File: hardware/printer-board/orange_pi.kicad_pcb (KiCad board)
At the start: 2 copper layers, 12 parts, among them J1 USB_DEBUG, U1 orange_pi_zero

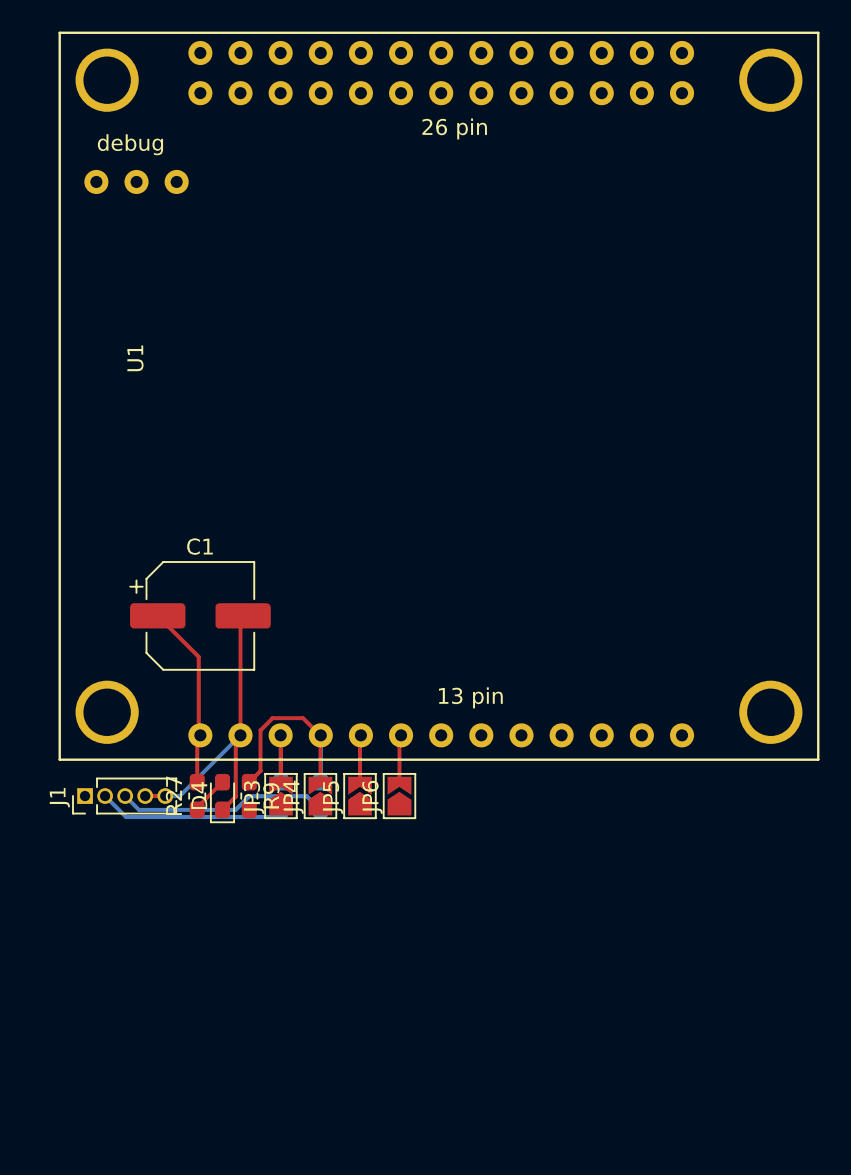
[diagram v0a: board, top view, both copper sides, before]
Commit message: update,
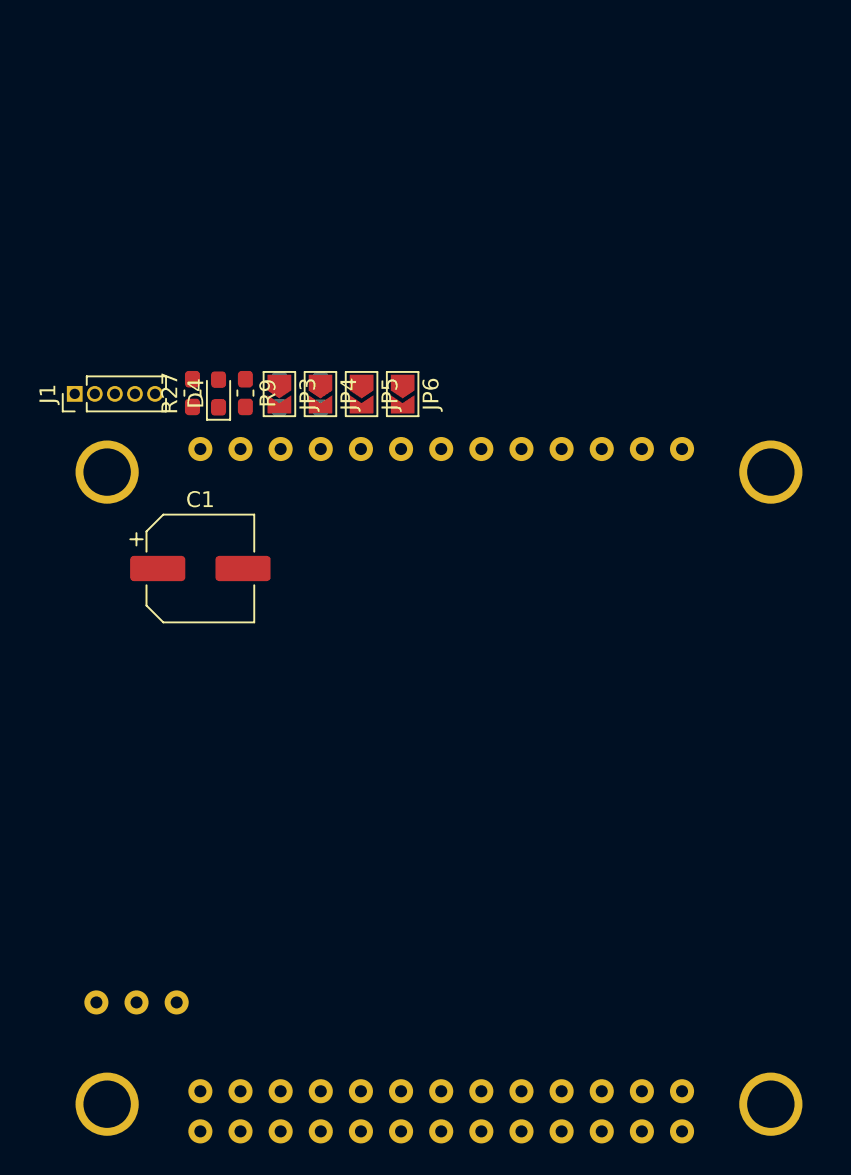
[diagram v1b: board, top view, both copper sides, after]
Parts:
- U1: moved to B.Cu
- moved R27 25.5 mm to (40.5, 46.4)
- moved R9 25.5 mm to (43.9, 46.4)
- moved D4 25.5 mm to (42.1, 46.4)
- moved J1 25.5 mm to (33.0, 46.5)
- moved R5 25.5 mm to (46.0, 46.4), turned to 90 degrees
- moved JP6 25.4 mm to (53.8, 46.5), turned to 270 degrees
- moved JP5 25.4 mm to (51.2, 46.5), turned to 270 degrees
- moved JP3 25.4 mm to (46.0, 46.5), turned to 270 degrees
- moved R7 25.4 mm to (48.6, 46.5), turned to 90 degrees
- moved JP4 25.4 mm to (48.6, 46.5), turned to 270 degrees
- moved U1 21.2 mm to (80.1, 48.4), turned to 270 degrees
- moved C1 3.00 mm to (41.0, 57.5)
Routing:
- net GND: track 20.4 -> 0.00 mm
- net /USB-DP2: track 14.2 -> 0.00 mm
- net Net-(J1-Pad3): track 13.4 -> 0.00 mm
- net Net-(J1-Pad2): track 11.9 -> 0.00 mm
- net +5V_PI_SRC: track 11.7 -> 0.00 mm
- net /USB-DM2: track 6.10 -> 0.00 mm
- net /USB-DP3: track 3.16 -> 0.00 mm
- net /USB-DM3: track 3.14 -> 0.00 mm
- net Net-(D4-Pad2): track 2.41 -> 0.00 mm
